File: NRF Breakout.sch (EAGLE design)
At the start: 58 parts, among them Q1 BSS123, Q2 BSS123, Q3 BSS123, Q4 BSS123

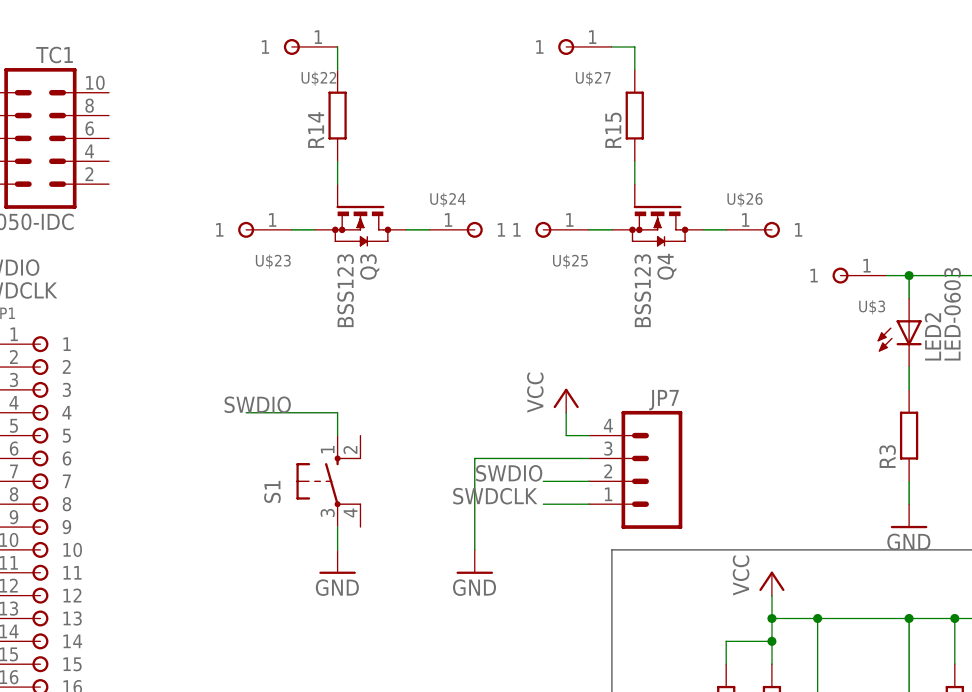
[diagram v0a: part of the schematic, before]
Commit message: Continued work. This is the version that was ordered from Seeed Studios.
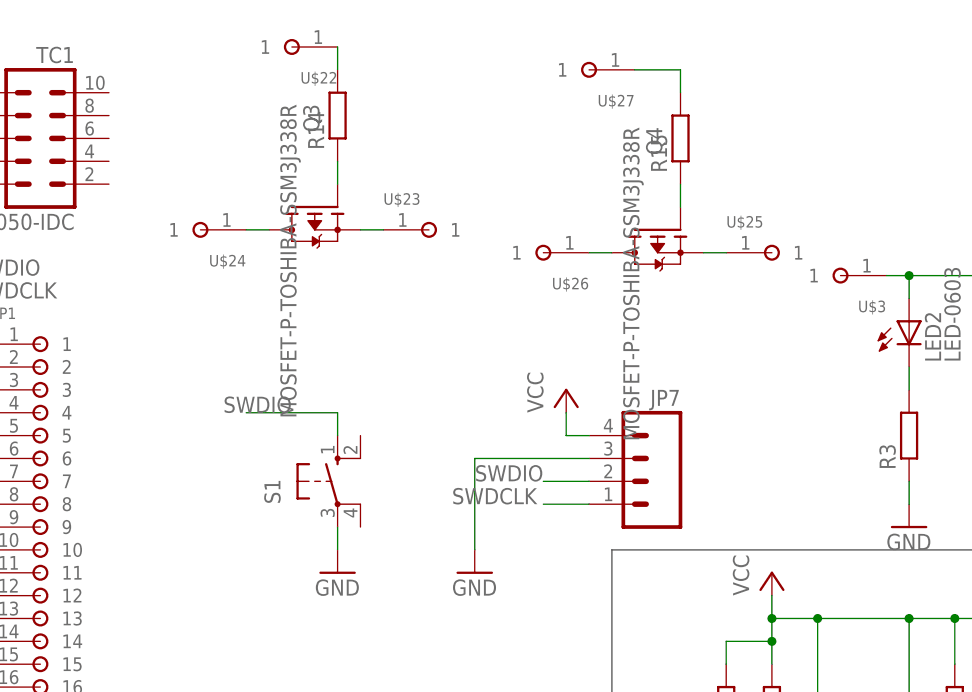
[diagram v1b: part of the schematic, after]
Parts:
- Q3, Q4: value BSS123 -> MOSFET-P-TOSHIBA-SSM3J338R; device Erland's Library:BSS123 -> Erland's Library:MOSFET-P-TOSHIBA-SSM3J338R
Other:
- moved on the sheet: R15, U$23, U$24, U$25, U$26, U$27
